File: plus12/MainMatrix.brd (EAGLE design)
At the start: 114.3 x 73.7 mm, 41 parts, among them SW1 RSTSWSMD, SW2 TRANSFERPADDY

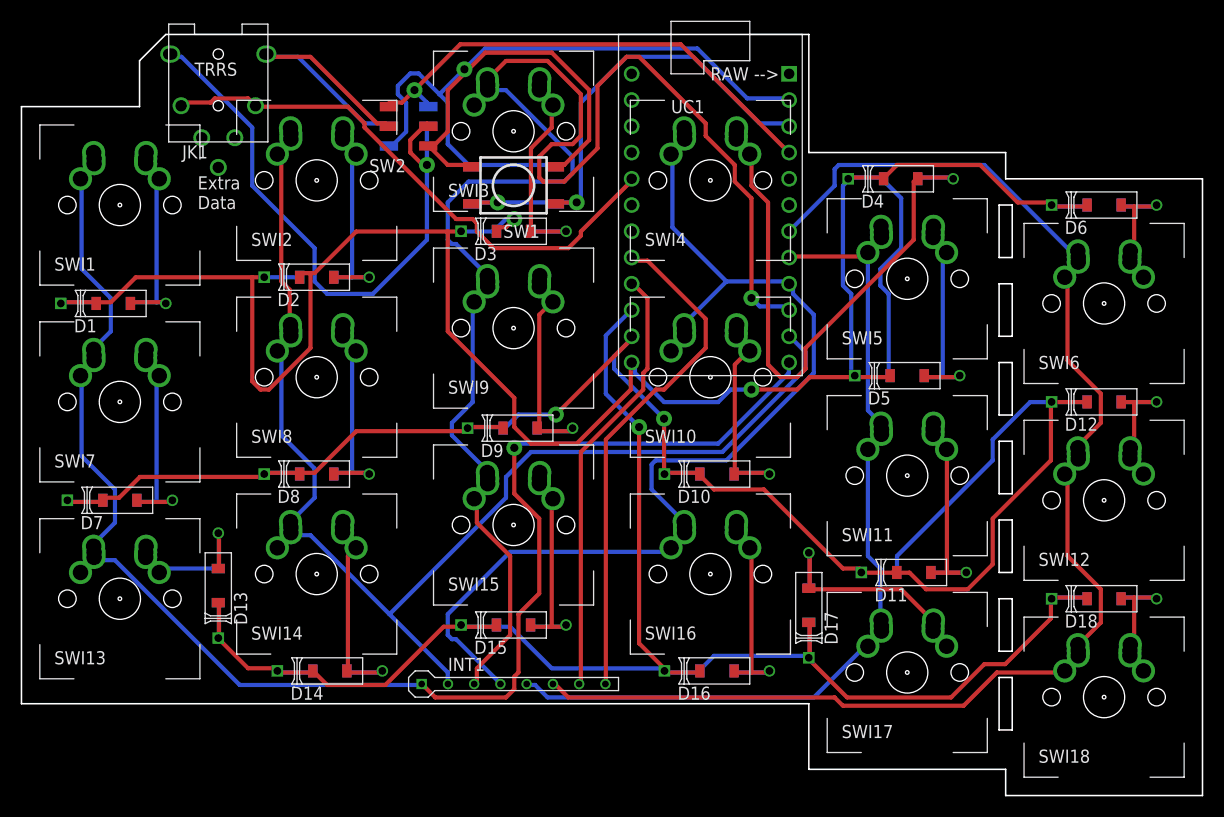
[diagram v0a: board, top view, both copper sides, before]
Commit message: Kobe beefing it up
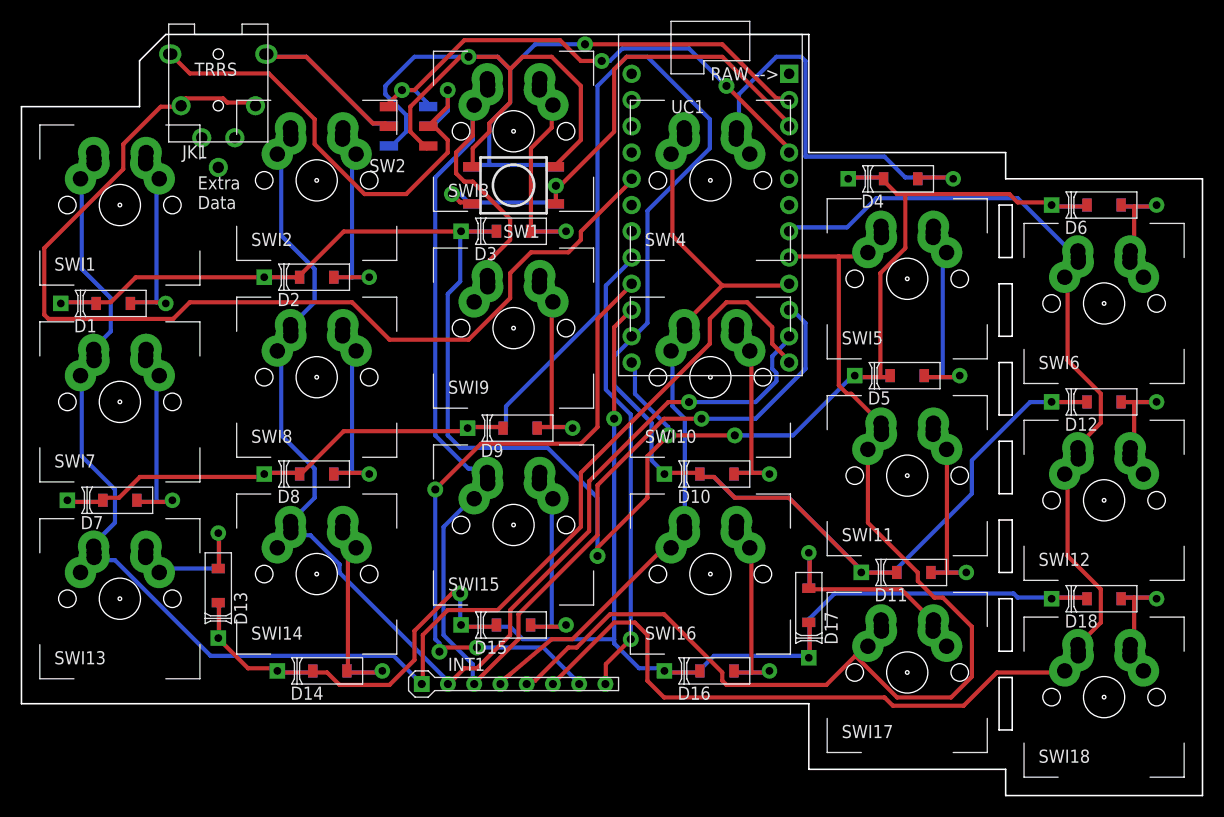
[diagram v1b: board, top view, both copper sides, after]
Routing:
- net N$21: track 178.2 -> 228.4 mm, vias 2 -> 0
- net N$32: track 53.9 -> 102.3 mm
- net N$26: track 107.9 -> 76.4 mm
- net N$1: track 90.8 -> 121.8 mm
- net N$29: track 42.1 -> 64.5 mm, vias 0 -> 3
- net N$20: track 218.2 -> 199.4 mm, vias 2 -> 3
- net N$5: track 55.7 -> 39.7 mm
- net N$30: track 59.3 -> 48.5 mm
- net N$35: track 104.5 -> 115.3 mm, vias 1 -> 2
- net N$25: track 159.7 -> 150.1 mm
- net N$33: track 49.4 -> 44.3 mm, vias 0 -> 1
- net N$22: track 164.3 -> 159.6 mm, vias 1 -> 2
- net N$28: track 47.9 -> 51.2 mm, vias 1 -> 3
- net N$23: track 153.1 -> 150.0 mm, vias 1 -> 0
- net N$27: track 139.1 -> 142.1 mm
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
